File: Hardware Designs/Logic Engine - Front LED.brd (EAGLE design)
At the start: 59.4 x 38.6 mm, 106 parts

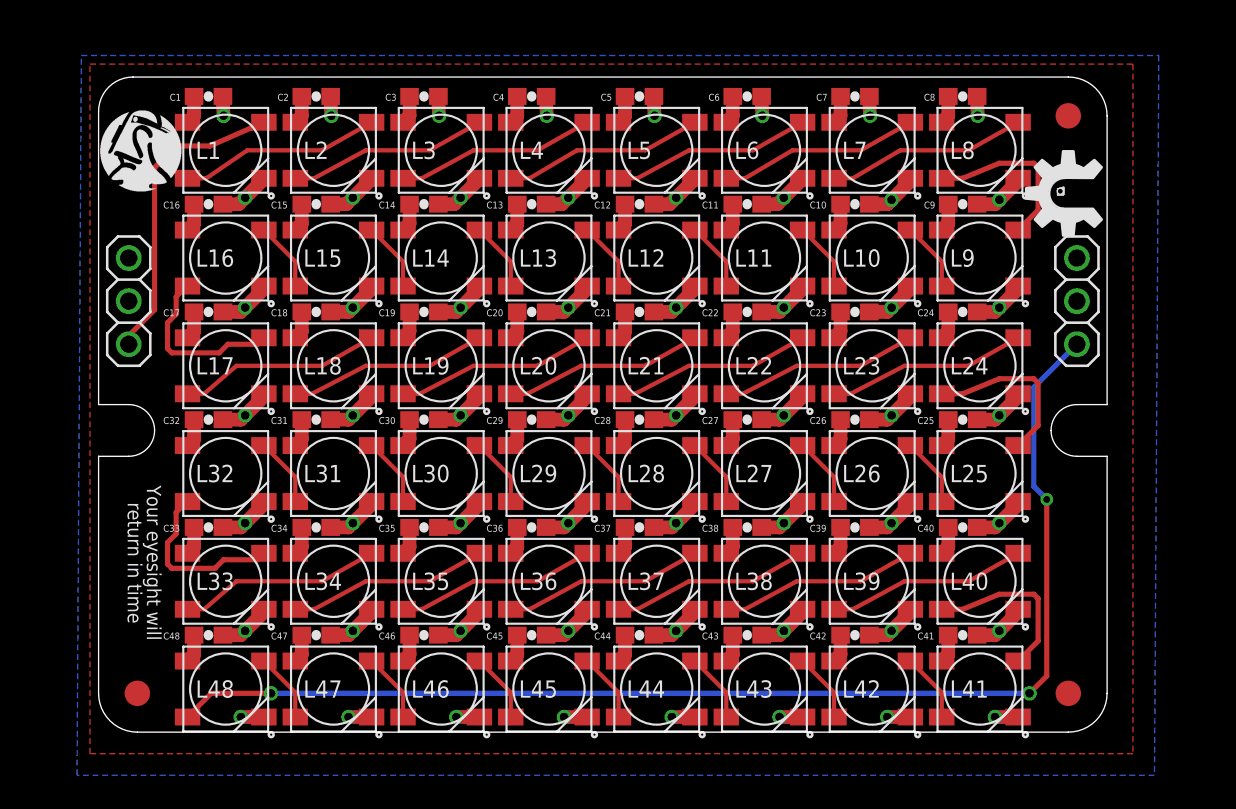
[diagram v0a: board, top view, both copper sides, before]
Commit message: updated Front LED board to current version
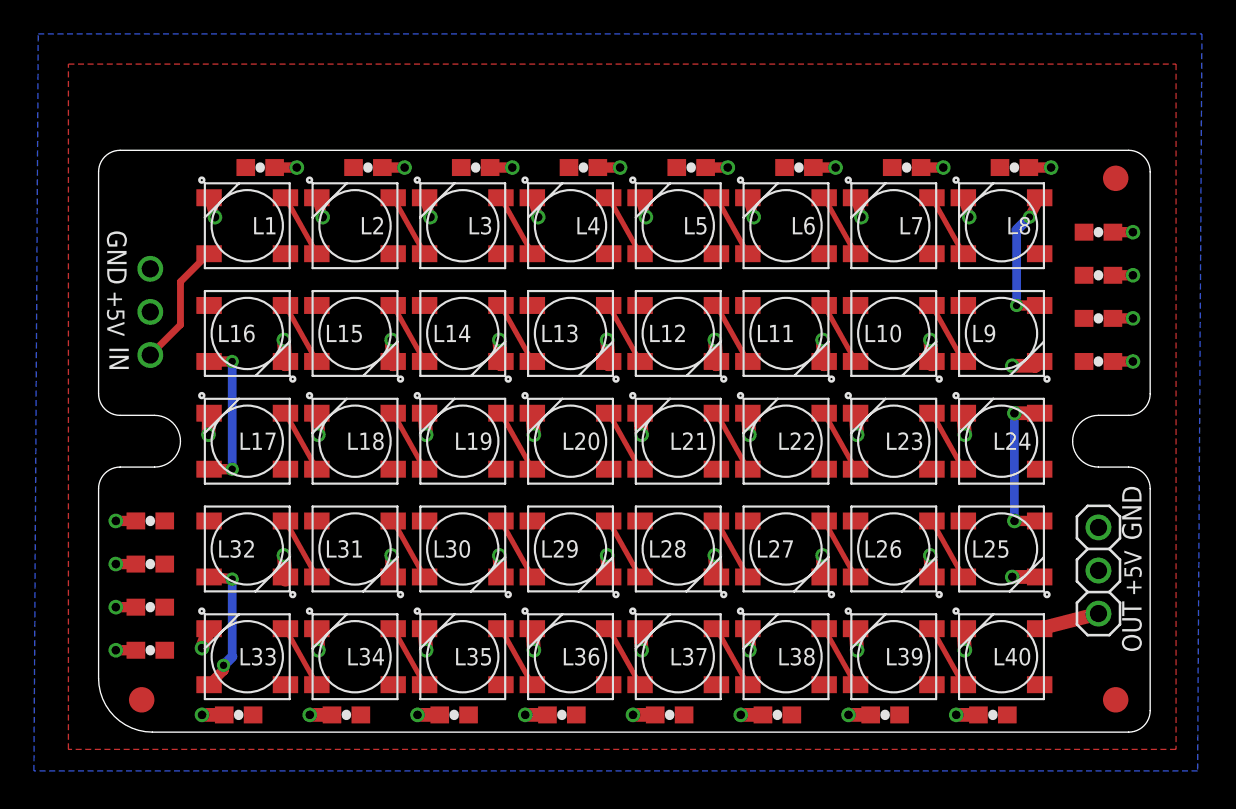
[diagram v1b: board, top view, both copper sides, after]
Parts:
- removed C14, C15, C16, C17, C18, C19, C20, C21, C22, C23, C26, C27, C28, C29, C30, C31, C41, C42, C43, C44, C45, C46, C47, C48: 0.1uF, SparkFun-Capacitors:0603-CAP
- removed L41, L42, L43, L44, L45, L46, L47, L48: WS2812B, rseries:WS2812B
- removed U$1: (no value), rseries:ROYAL-ENGINEERS-OF-NABOO-BOTTOM-LARGE
- removed U$3: (no value), rseries:RSERIES-OSHW-LOGO-MEDIUM-BOTTOM
- removed U$4, U$5: (no value), rseries:R2BUILDERS-LOGO
- U$2: device rseries:RSERIES-OSHW-LOGO-MEDIUM-BOTTOM -> rseries:R2BUILDERS-LOGO
- moved U$2 63.4 mm to (0.51, 5.46), flipped to the bottom, turned to 180 degrees
- moved C10 45.5 mm to (3.05, 12.4), turned to 180 degrees
- moved C11 42.4 mm to (3.05, 7.37), turned to 180 degrees
- moved C13 30.9 mm to (3.05, 9.91), turned to 180 degrees
- moved C12 28.6 mm to (58.9, 21.8)
- moved OUT 15.9 mm to (58.9, 9.53)
- moved C32 14.0 mm to (3.05, 4.83), turned to 180 degrees
- moved C33 11.2 mm to (8.26, 1.02), turned to 180 degrees
- moved C34 11.2 mm to (14.6, 1.02), turned to 180 degrees
- moved C37 11.2 mm to (33.7, 1.02), turned to 180 degrees
- moved C38 11.2 mm to (40.0, 1.02), turned to 180 degrees
- moved C35 11.2 mm to (21.0, 1.02), turned to 180 degrees
- moved C36 11.2 mm to (27.3, 1.02), turned to 180 degrees
- moved C39 11.2 mm to (46.4, 1.02), turned to 180 degrees
- moved C40 11.2 mm to (52.7, 1.02), turned to 180 degrees
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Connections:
- removed net N$33: L41.DOUT, L42.DIN
- removed net N$34: L42.DOUT, L43.DIN
- removed net N$35: L43.DOUT, L44.DIN
- removed net N$36: L44.DOUT, L45.DIN
- removed net N$37: L45.DOUT, L46.DIN
- removed net N$38: L46.DOUT, L47.DIN
- removed net N$39: L47.DOUT, L48.DIN
- removed net N$47: L40.DOUT, L41.DIN
- net +5V: no longer C14.1, C15.1, C16.1, C17.1, C18.1, C19.1, C20.1, C21.1, C22.1, C23.1, C26.1, C27.1, C28.1, C29.1, C30.1, C31.1, C41.1, C42.1, C43.1, C44.1, C45.1, C46.1, C47.1, C48.1, L41.VDD, L42.VDD, L43.VDD, L44.VDD, L45.VDD, L46.VDD, L47.VDD, L48.VDD
- net DOUT: now also L40.DOUT; no longer L48.DOUT
- net GND: no longer C14.2, C15.2, C16.2, C17.2, C18.2, C19.2, C20.2, C21.2, C22.2, C23.2, C26.2, C27.2, C28.2, C29.2, C30.2, C31.2, C41.2, C42.2, C43.2, C44.2, C45.2, C46.2, C47.2, C48.2, L41.VSS, L42.VSS, L43.VSS, L44.VSS, L45.VSS, L46.VSS, L47.VSS, L48.VSS
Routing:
- net +5V: track 80.8 -> 0.00 mm
- net DOUT: track 72.6 -> 3.58 mm, vias 3 -> 0
- net GND: track 145.3 -> 83.8 mm, vias 56 -> 64
- net DIN: track 18.3 -> 7.43 mm
- net N$47: track 10.1 -> 0.00 mm
- net N$22: track 11.9 -> 3.78 mm
- net N$8: track 11.9 -> 3.78 mm
- net N$40: track 11.8 -> 3.78 mm
- net N$45: track 11.7 -> 3.78 mm
- net N$43: track 11.7 -> 3.78 mm
- net N$46: track 11.7 -> 3.78 mm
- net N$44: track 11.7 -> 3.78 mm
- net N$41: track 11.7 -> 3.78 mm
- net N$27: track 11.7 -> 3.78 mm
- net N$26: track 11.7 -> 3.78 mm
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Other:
- board size 59.4 x 38.6 mm -> 62 x 34.3 mm
- board text added: "+5V"
- board text added: "GND"
- board text added: "IN"
- board text added: "OUT"
- board text added: "Paul Murphy 20150302"
- board text added: "RSeries Logic Engine"
- board text removed: "+ -"
- board text removed: "RSeries Logic Engine LED Board : 2013-11-24"
- board text removed: "Your eyesight will return in time"
